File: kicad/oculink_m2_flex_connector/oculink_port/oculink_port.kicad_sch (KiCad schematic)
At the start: 8 parts, among them J1 G14A42121B12HR, J2 Conn_01x38_Pin

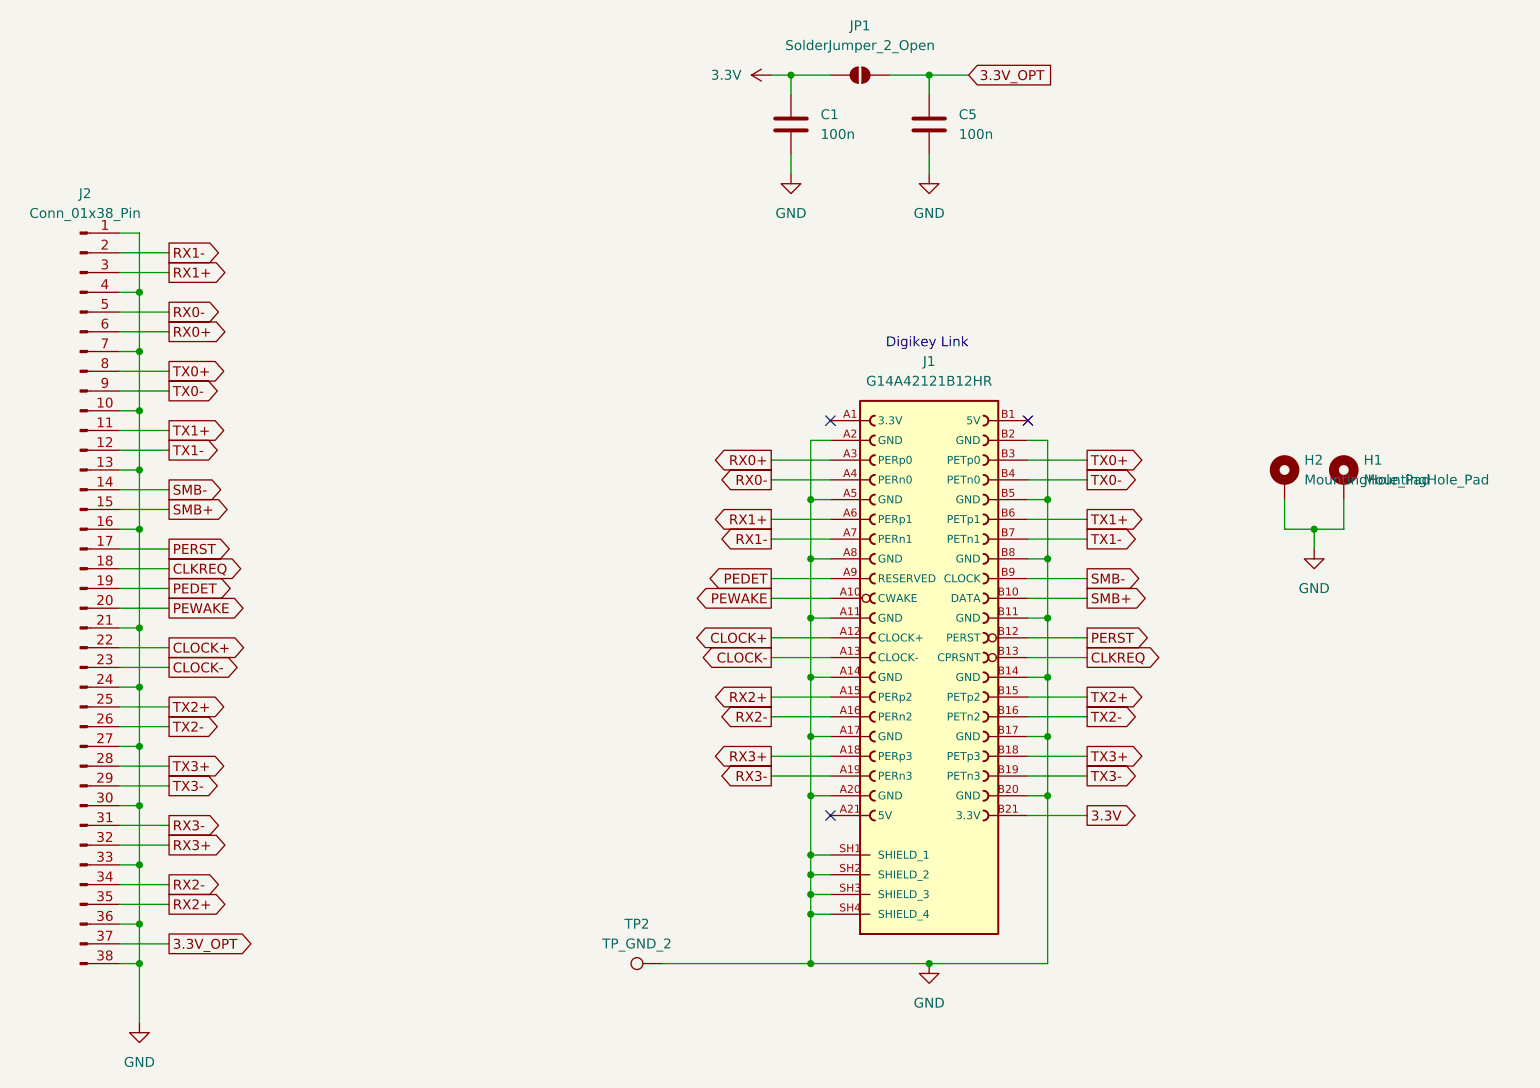
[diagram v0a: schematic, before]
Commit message: Initial layout of port side board
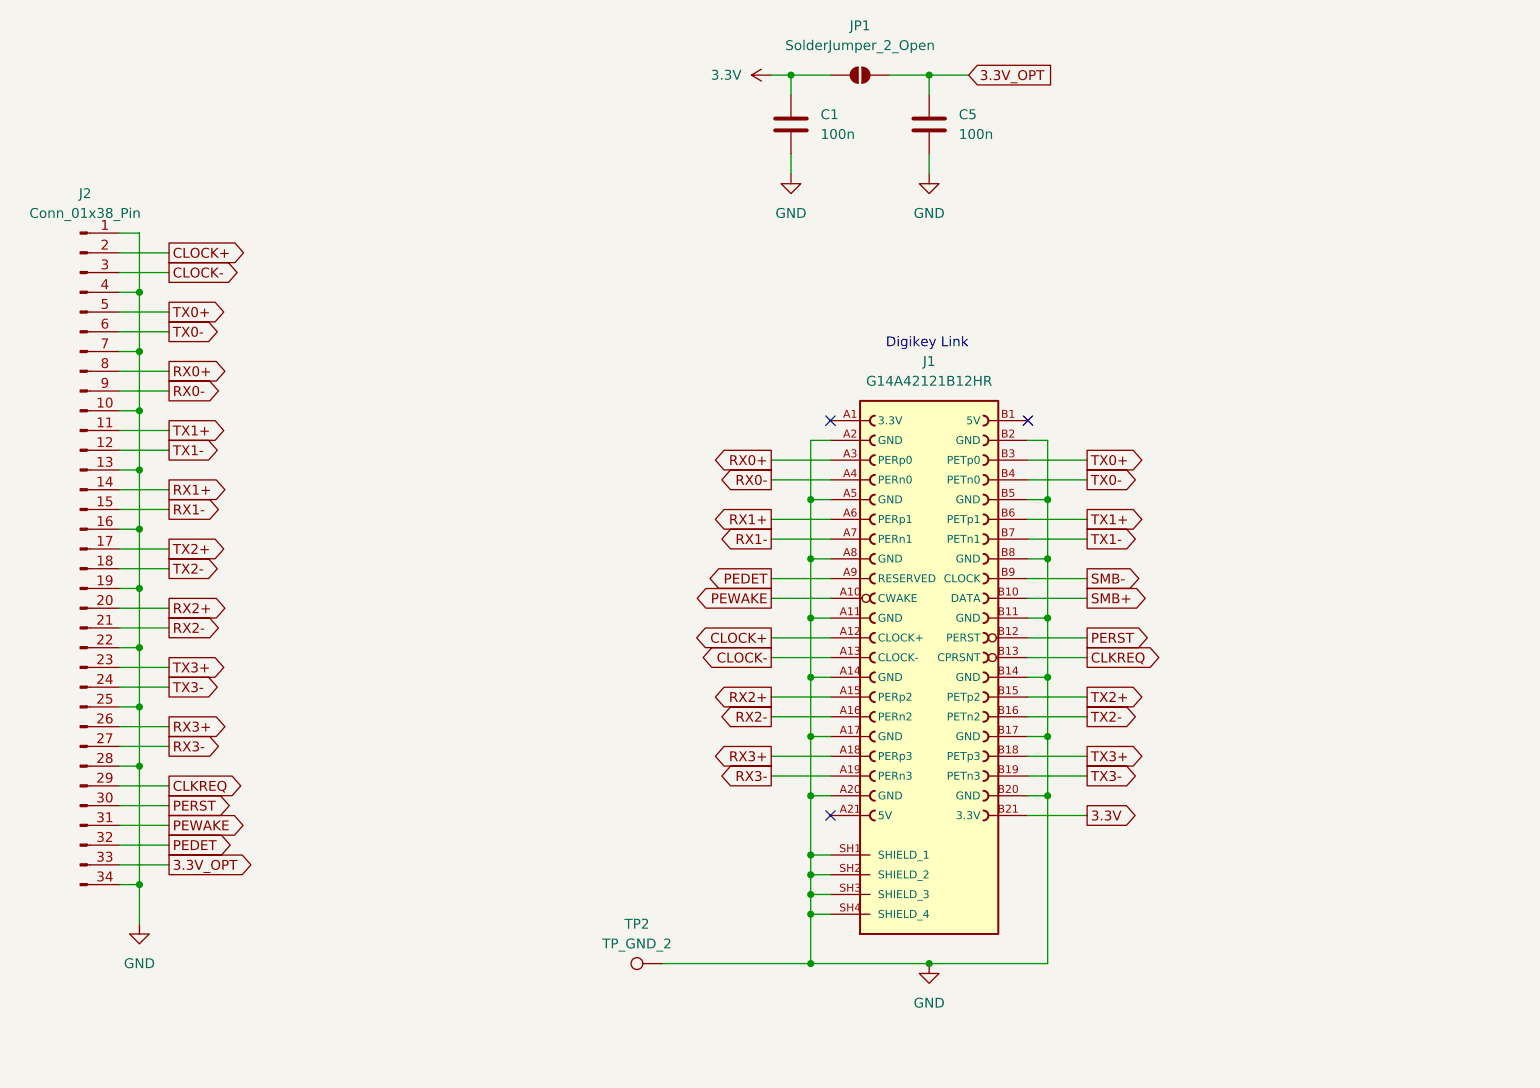
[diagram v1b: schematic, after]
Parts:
- removed H1, H2: MountingHole_Pad, custom:mounting_pad_1mm, symbol Mechanical:MountingHole_Pad
- removed J2: Conn_01x38_Pin, flex_connector:port_pcb, symbol Connector:Conn_01x38_Pin
- added J2: Conn_01x38_Pin, flex_connector:port_pcb, symbol Connector:Conn_01x34_Pin
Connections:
- net 3.3V_OPT: now also J2.33 (Pin_33)
- net CLKREQ: now also J2.29 (Pin_29)
- net CLOCK+: now also J2.2 (Pin_2)
- net CLOCK-: now also J2.3 (Pin_3)
- net GND: now also J2.1 (Pin_1), J2.10 (Pin_10), J2.13 (Pin_13), J2.16 (Pin_16), J2.19 (Pin_19), J2.22 (Pin_22), J2.25 (Pin_25), J2.28 (Pin_28), J2.34 (Pin_34), J2.4 (Pin_4), J2.7 (Pin_7)
- net PEDET: now also J2.32 (Pin_32)
- net PERST: now also J2.30 (Pin_30)
- net PEWAKE: now also J2.31 (Pin_31)
- net RX0+: now also J2.8 (Pin_8)
- net RX0-: now also J2.9 (Pin_9)
- net RX1+: now also J2.14 (Pin_14)
- net RX1-: now also J2.15 (Pin_15)
- net RX2+: now also J2.20 (Pin_20)
- net RX2-: now also J2.21 (Pin_21)
- net RX3+: now also J2.26 (Pin_26)
- net RX3-: now also J2.27 (Pin_27)
- net TX0+: now also J2.5 (Pin_5)
- net TX0-: now also J2.6 (Pin_6)
- net TX1+: now also J2.11 (Pin_11)
- net TX1-: now also J2.12 (Pin_12)
- net TX2+: now also J2.17 (Pin_17)
- net TX2-: now also J2.18 (Pin_18)
- net TX3+: now also J2.23 (Pin_23)
- net TX3-: now also J2.24 (Pin_24)
